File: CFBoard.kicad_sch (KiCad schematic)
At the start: 19 parts, among them SW1 Slide Switch, U1 STM32 Blue Pill, U2 Wemos D1 Mini, U3 GY-6500, U4 BMP180_5pin

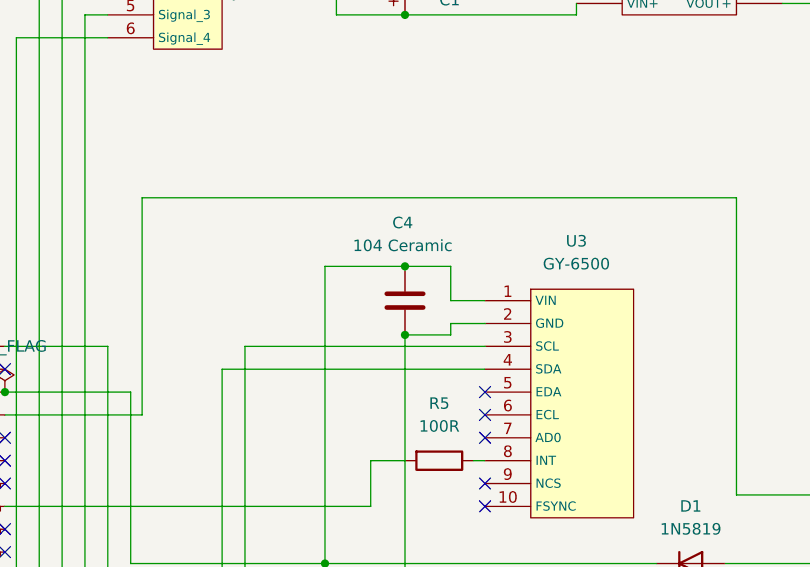
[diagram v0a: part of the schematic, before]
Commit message: feat: update design
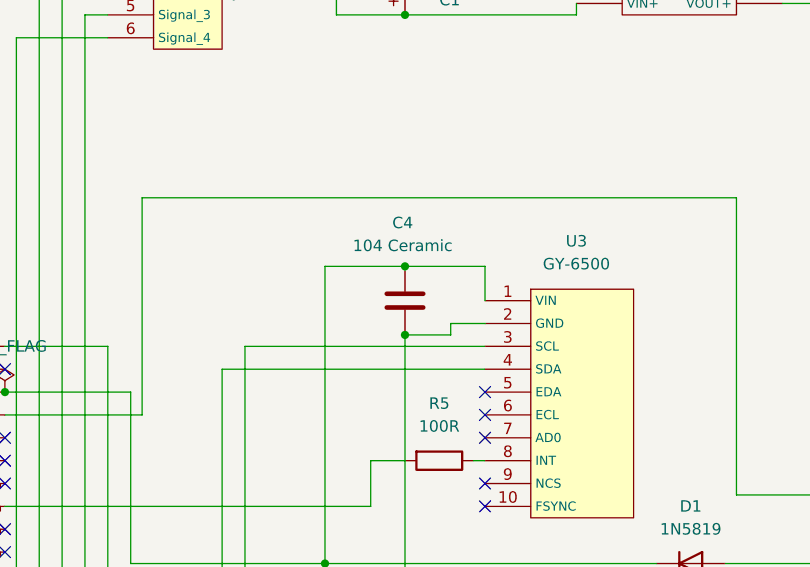
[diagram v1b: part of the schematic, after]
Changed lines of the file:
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@@
+	(wire
+		(pts
+			(xy 151.13 76.2) (xy 160.02 76.2)
+		)
+		(stroke
+			(width 0)
+			(type default)
+		)
+	)
 	(wire
 		(pts
@@
 	(wire
 		(pts
-			(xy 160.02 80.01) (xy 156.21 80.01)
-		)
-		(stroke
-			(width 0)
-			(type default)
-		)
-	)
-	(wire
-		(pts
 			(xy 142.24 134.62) (xy 151.13 134.62)
 		)
@@
 	(wire
 		(pts
-			(xy 156.21 76.2) (xy 151.13 76.2)
-		)
-		(stroke
-			(width 0)
-			(type default)
-		)
-	)
-	(wire
-		(pts
 			(xy 213.36 111.76) (xy 213.36 109.22)
 		)
@@
 	(wire
 		(pts
+			(xy 160.02 76.2) (xy 160.02 80.01)
+		)
+		(stroke
+			(width 0)
+			(type default)
+		)
+	)
+	(wire
+		(pts
 			(xy 133.35 85.09) (xy 133.35 137.16)
 		)
@@
 	(wire
 		(pts
+			(xy 142.24 76.2) (xy 151.13 76.2)
+		)
+		(stroke
+			(width 0)
+			(type default)
+		)
+	)
+	(wire
+		(pts
 			(xy 232.41 129.54) (xy 237.49 129.54)
 		)
@@
 	(wire
 		(pts
-			(xy 151.13 76.2) (xy 142.24 76.2)
-		)
-		(stroke
-			(width 0)
-			(type default)
-		)
-	)
-	(wire
-		(pts
 			(xy 118.11 40.64) (xy 114.3 40.64)
 		)
 		(stroke
-			(width 0)
-			(type default)
-		)
-	)
-	(wire
-		(pts
-			(xy 156.21 80.01) (xy 156.21 76.2)
-		)
-		(stroke

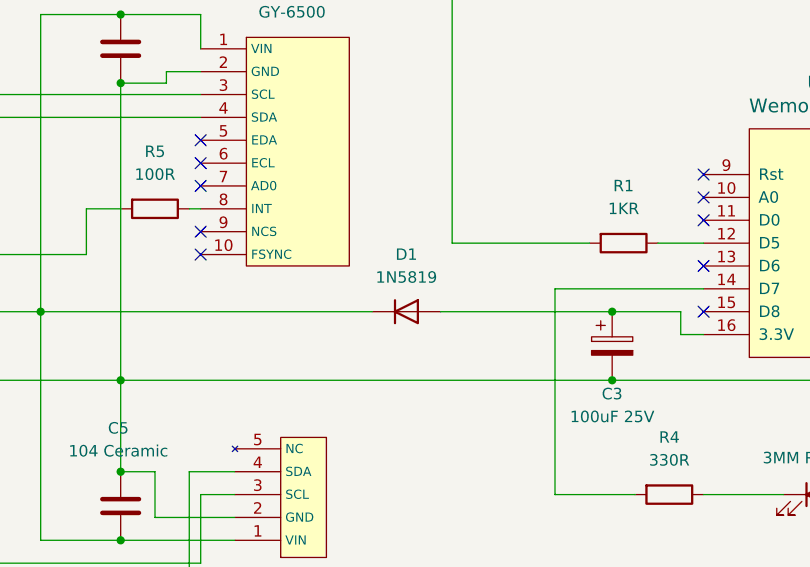
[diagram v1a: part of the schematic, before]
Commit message: feat: update jst connector footprint design
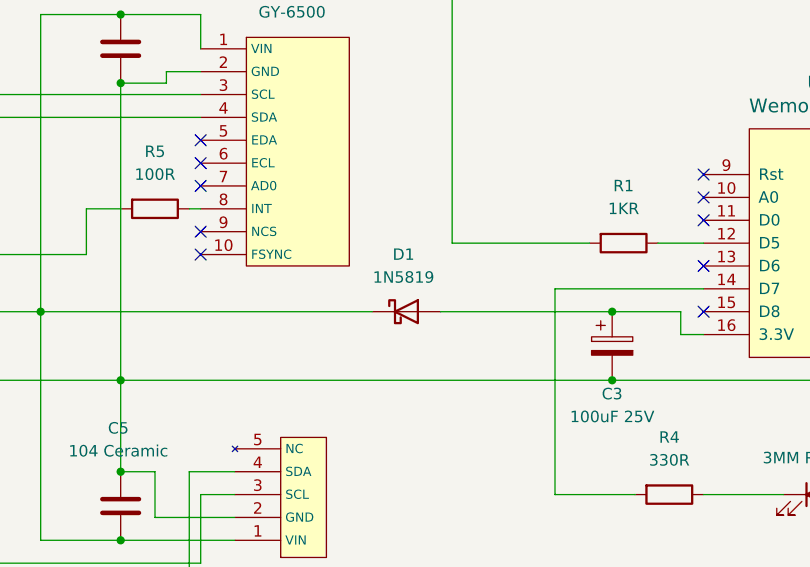
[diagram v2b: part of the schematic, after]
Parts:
- removed D1: 1N5819, Diode_THT:D_DO-41_SOD81_P7.62mm_Horizontal, symbol Device:D
- added D1: 1N5819, Diode_THT:D_DO-41_SOD81_P10.16mm_Horizontal, symbol Diode:1N5819
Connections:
- net at C3.1, U2.16 (3.3V): now also D1.2 (A)
- net at C4.1, C5.2, U1.38 (3V3)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: now also D1.1 (K)
